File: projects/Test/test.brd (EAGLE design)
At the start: 63.5 x 24.1 mm, 47 parts, among them J2 1755529, U1 STM32F405RGT6, U2 CSD88584Q5DCT, U3 CSD88584Q5DCT, U4 CSD88584Q5DCT, Y1 ECS-80-S-4X

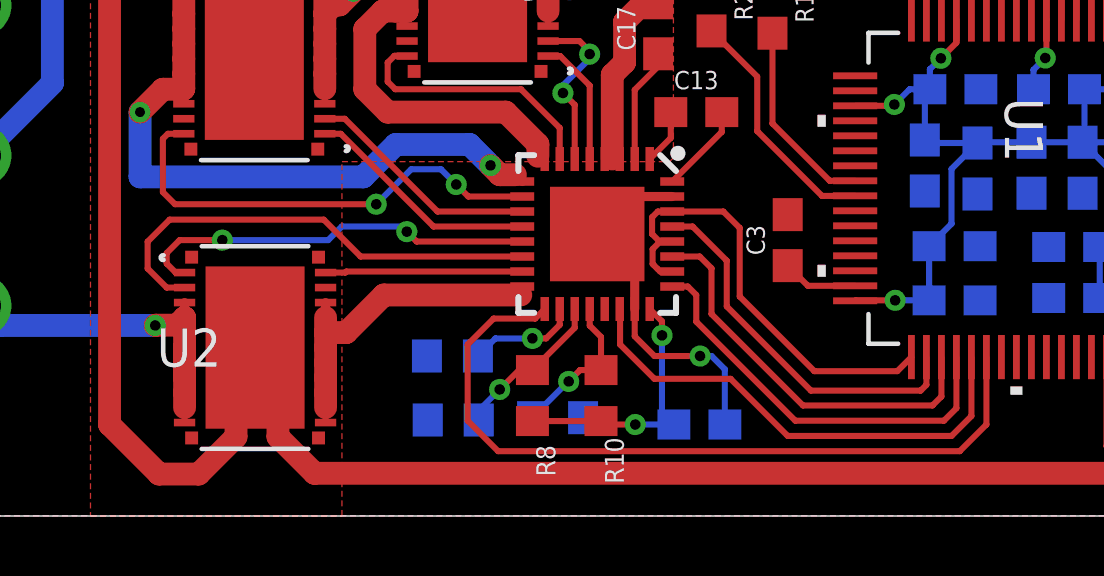
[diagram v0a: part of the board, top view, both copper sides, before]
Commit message: fixed(?) some stuff on the board
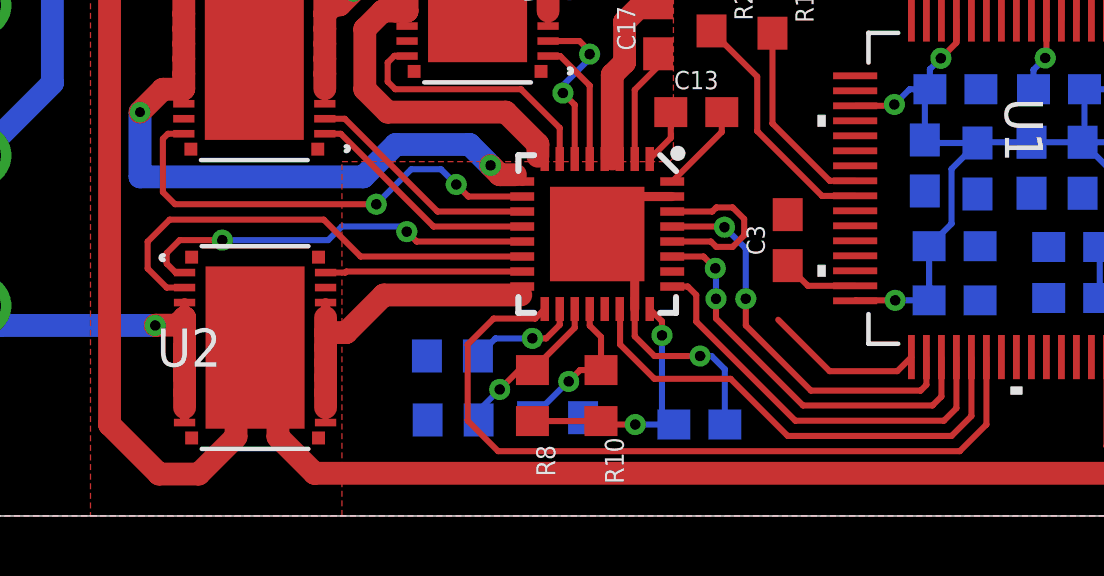
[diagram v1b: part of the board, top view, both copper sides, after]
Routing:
- net INL_1: track 15.4 -> 11.1 mm
- net INHC_1: track 12.6 -> 13.2 mm, vias 0 -> 2
- net INHB_1: vias 0 -> 2
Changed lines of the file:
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@@
 <?xml version="1.0" encoding="utf-8"?>
 <!DOCTYPE eagle SYSTEM "eagle.dtd">
-<eagle version="9.5.1">
+<eagle version="9.4.1">
 <drawing>
 <settings>
@@
 <wire x1="6.2484" y1="6.35" x2="5.588" y2="7.0104" width="0.762" layer="16"/>
 <wire x1="12.4074" y1="6.6134" x2="12.4074" y2="7.1134" width="0.3048" layer="1"/>
-<wire x1="12.4074" y1="3.1134" x2="12.4074" y2="3.6134" width="0.2032" layer="1"/>
+<wire x1="12.4074" y1="3.175" x2="12.4074" y2="3.6134" width="0.3048" layer="1"/>
+<wire x1="12.4074" y1="3.1134" x2="12.4074" y2="3.175" width="0.2032" layer="1"/>
 </signal>
 <signal name="12V">
@@
 <wire x1="37.636" y1="3.981" x2="37.338" y2="3.683" width="0.2032" layer="1"/>
 <wire x1="37.338" y1="3.683" x2="33.02" y2="3.683" width="0.2032" layer="1"/>
-<wire x1="29.579" y1="8.648" x2="29.972" y2="8.255" width="0.2032" layer="1"/>
-<wire x1="33.02" y1="3.683" x2="29.972" y2="6.731" width="0.2032" layer="1"/>
-<wire x1="29.972" y1="6.731" x2="29.972" y2="8.255" width="0.2032" layer="1"/>
-<wire x1="28.662" y1="8.648" x2="29.579" y2="8.648" width="0.2032" layer="1"/>
+<wire x1="33.02" y1="3.683" x2="30.1216" y2="6.5814" width="0.2032" layer="1"/>
+<wire x1="28.662" y1="8.648" x2="29.706" y2="8.648" width="0.2032" layer="1"/>
+<wire x1="29.706" y1="8.648" x2="30.099" y2="8.255" width="0.2032" layer="1"/>
+<via x="30.099" y="8.255" extent="1-16" drill="0.35"/>
+<wire x1="30.099" y1="8.255" x2="30.1216" y2="8.2324" width="0.2032" layer="16"/>
+<wire x1="30.1216" y1="8.2324" x2="30.1216" y2="7.239" width="0.2032" layer="16"/>
+<via x="30.1216" y="7.239" extent="1-16" drill="0.35"/>
+<wire x1="30.1216" y1="7.239" x2="30.1216" y2="6.5814" width="0.2032" layer="1"/>
 </signal>
 <signal name="INL_1">
@@
 <contactref element="U$2" pad="30"/>
 <contactref element="U$2" pad="28"/>
-<wire x1="28.662" y1="10.148" x2="30.365" y2="10.148" width="0.2032" layer="1"/>
-<wire x1="30.365" y1="10.148" x2="30.9118" y2="9.6012" width="0.2032" layer="1"/>
-<wire x1="30.9118" y1="7.3152" x2="33.401" y2="4.826" width="0.2032" layer="1"/>
-<wire x1="33.401" y1="4.826" x2="36.1661" y2="4.826" width="0.2032" layer="1"/>
+<wire x1="32.1945" y1="6.5405" x2="33.909" y2="4.826" width="0.2032" layer="1"/>
+<wire x1="33.909" y1="4.826" x2="36.1661" y2="4.826" width="0.2032" layer="1"/>
 <wire x1="36.1661" y1="4.826" x2="36.636" y2="5.2959" width="0.2032" layer="1"/>
-<wire x1="30.9118" y1="9.6012" x2="30.9118" y2="7.3152" width="0.2032" layer="1"/>
-<wire x1="28.662" y1="10.148" x2="28.182" y2="10.148" width="0.2032" layer="1"/>
-<wire x1="27.991" y1="9.957" x2="27.991" y2="9.398" width="0.2032" layer="1"/>
-<wire x1="27.991" y1="9.398" x2="28.241" y2="9.148" width="0.2032" layer="1"/>
-<wire x1="28.241" y1="9.148" x2="28.662" y2="9.148" width="0.2032" layer="1"/>
-<wire x1="28.182" y1="10.148" x2="27.991" y2="9.957" width="0.2032" layer="1"/>
-<wire x1="28.008" y1="8.4004875" x2="28.008" y2="8.8955125" width="0.2032" layer="1"/>
-<wire x1="28.241" y1="9.1285125" x2="28.241" y2="9.148" width="0.2032" layer="1"/>
-<wire x1="28.008" y1="8.8955125" x2="28.241" y2="9.1285125" width="0.2032" layer="1"/>
-<wire x1="28.1668875" y1="8.2416" x2="28.04674375" y2="8.36174375" width="0.2032" layer="1"/>
-<wire x1="28.04674375" y1="8.36174375" x2="28.008" y2="8.4004875" width="0.2032" layer="1"/>
-<wire x1="28.662" y1="8.148" x2="28.2604875" y2="8.148" width="0.2032" layer="1"/>
-<wire x1="28.2604875" y1="8.148" x2="28.1668875" y2="8.2416" width="0.2032" layer="1"/>
+<wire x1="30.1314125" y1="8.969" x2="30.6761875" y2="8.969" width="0.2032" layer="1"/>
+<wire x1="30.6761875" y1="8.969" x2="31.0614" y2="9.3542125" width="0.2032" layer="1"/>
+<wire x1="31.0614" y1="9.3542125" x2="31.0614" y2="9.8989875" width="0.2032" layer="1"/>
+<wire x1="31.0614" y1="9.8989875" x2="30.6761875" y2="10.2842" width="0.2032" layer="1"/>
+<wire x1="30.6761875" y1="10.2842" x2="30.1314125" y2="10.2842" width="0.2032" layer="1"/>
+<wire x1="28.662" y1="9.148" x2="29.9524125" y2="9.148" width="0.2032" layer="1"/>
+<wire x1="29.9524125" y1="9.148" x2="30.1314125" y2="8.969" width="0.2032" layer="1"/>
+<wire x1="30.1314125" y1="10.2842" x2="29.9952125" y2="10.148" width="0.2032" layer="1"/>
+<wire x1="29.9952125" y1="10.148" x2="28.662" y2="10.148" width="0.2032" layer="1"/>
+<wire x1="28.662" y1="9.148" x2="28.662" y2="8.148" width="0" layer="19" extent="1-1"/>
+<wire x1="28.662" y1="10.148" x2="32.1945" y2="6.5405" width="0" layer="19" extent="1-1"/>
 </signal>
 <signal name="INHC_1">
 <contactref element="U1" pad="34"/>
 <contactref element="U$2" pad="29"/>
-<wire x1="30.48" y1="8.509" x2="29.341" y2="9.648" width="0.2032" layer="1"/>
 <wire x1="37.136" y1="5.2959" x2="37.136" y2="4.37" width="0.2032" layer="1"/>
-<wire x1="36.9443" y1="4.1783" x2="33.2867" y2="4.1783" width="0.2032" layer="1"/>
+<wire x1="33.2867" y1="4.1783" x2="36.9443" y2="4.1783" width="0.2032" layer="1"/>
 <wire x1="37.136" y1="4.37" x2="36.9443" y2="4.1783" width="0.2032" layer="1"/>
-<wire x1="33.2867" y1="4.1783" x2="30.48" y2="6.985" width="0.2032" layer="1"/>
-<wire x1="30.48" y1="6.985" x2="30.48" y2="8.509" width="0.2032" layer="1"/>
-<wire x1="29.341" y1="9.648" x2="28.662" y2="9.648" width="0.2032" layer="1"/>
+<wire x1="28.662" y1="9.648" x2="30.3824" y2="9.648" width="0.2032" layer="1"/>
+<wire x1="30.3824" y1="9.648" x2="30.4038" y2="9.6266" width="0.2032" layer="1"/>
+<via x="30.4038" y="9.6266" extent="1-16" drill="0.35"/>
+<wire x1="30.4038" y1="9.6266" x2="31.115" y2="8.9154" width="0.2032" layer="16"/>
+<wire x1="31.115" y1="8.9154" x2="31.115" y2="7.239" width="0.2032" layer="16"/>
+<via x="31.115" y="7.239" extent="1-16" drill="0.35"/>
+<wire x1="31.115" y1="7.239" x2="31.115" y2="6.35" width="0.2032" layer="1"/>
+<wire x1="31.115" y1="6.35" x2="33.2867" y2="4.1783" width="0.2032" layer="1"/>
 </signal>
 <signal name="OSC_IN">
